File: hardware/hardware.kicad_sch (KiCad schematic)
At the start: 53 parts, among them J1 SWD, J2 serial, J3 analog, J4 digital_0, J5 digital_1, J6 digital_2, J7 digital_3, J8 power_0, J9 power_1, SW1 reset_btn, SW2 user_btn, SW3 SW_SPDT, U1 STM32F030CCTx, U2 AMS1117-3.3, Y1 crystal

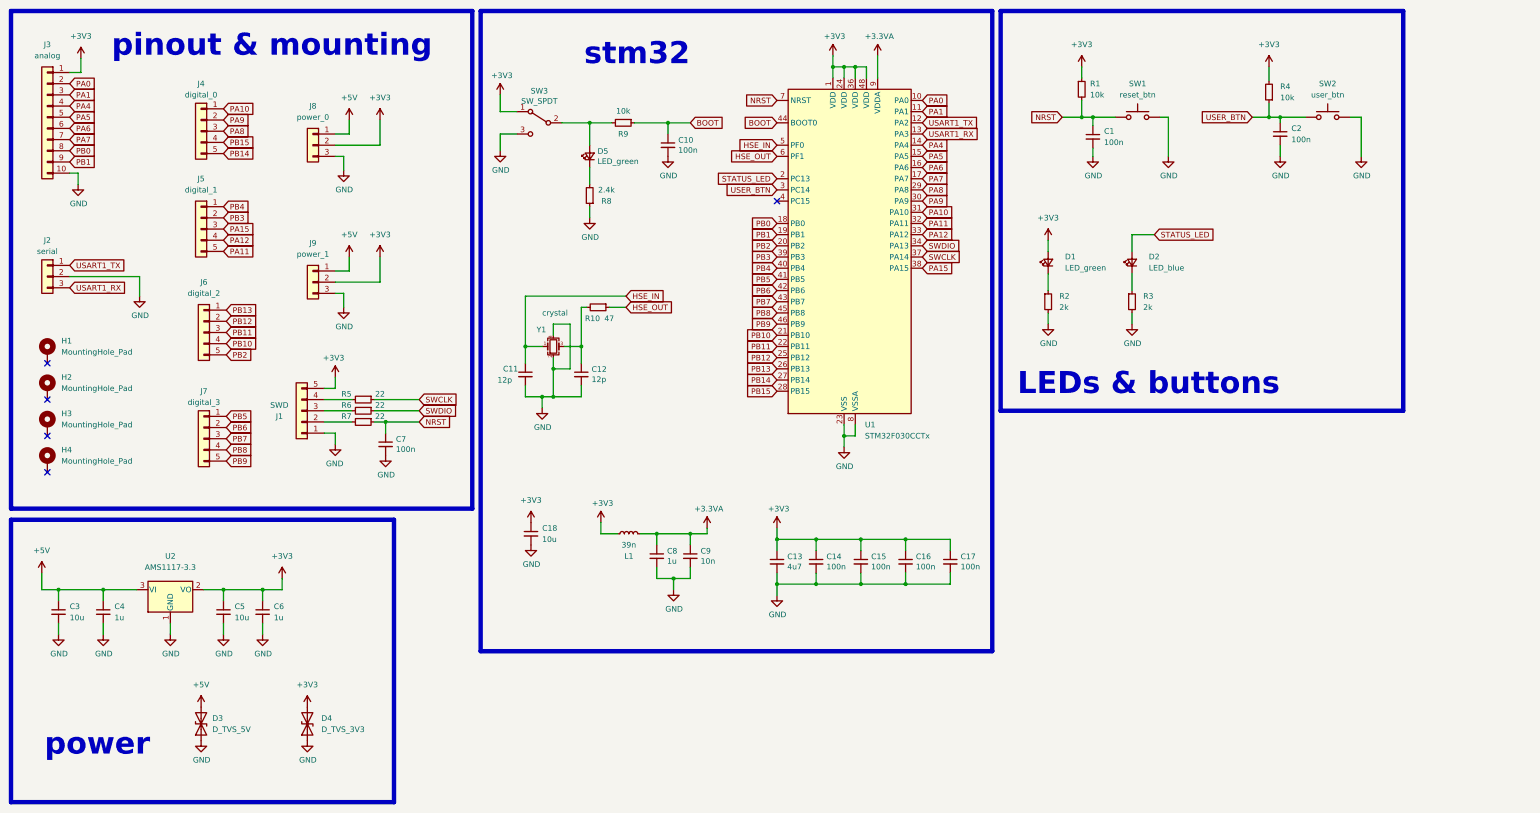
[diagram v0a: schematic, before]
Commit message: soldered and tested hardware
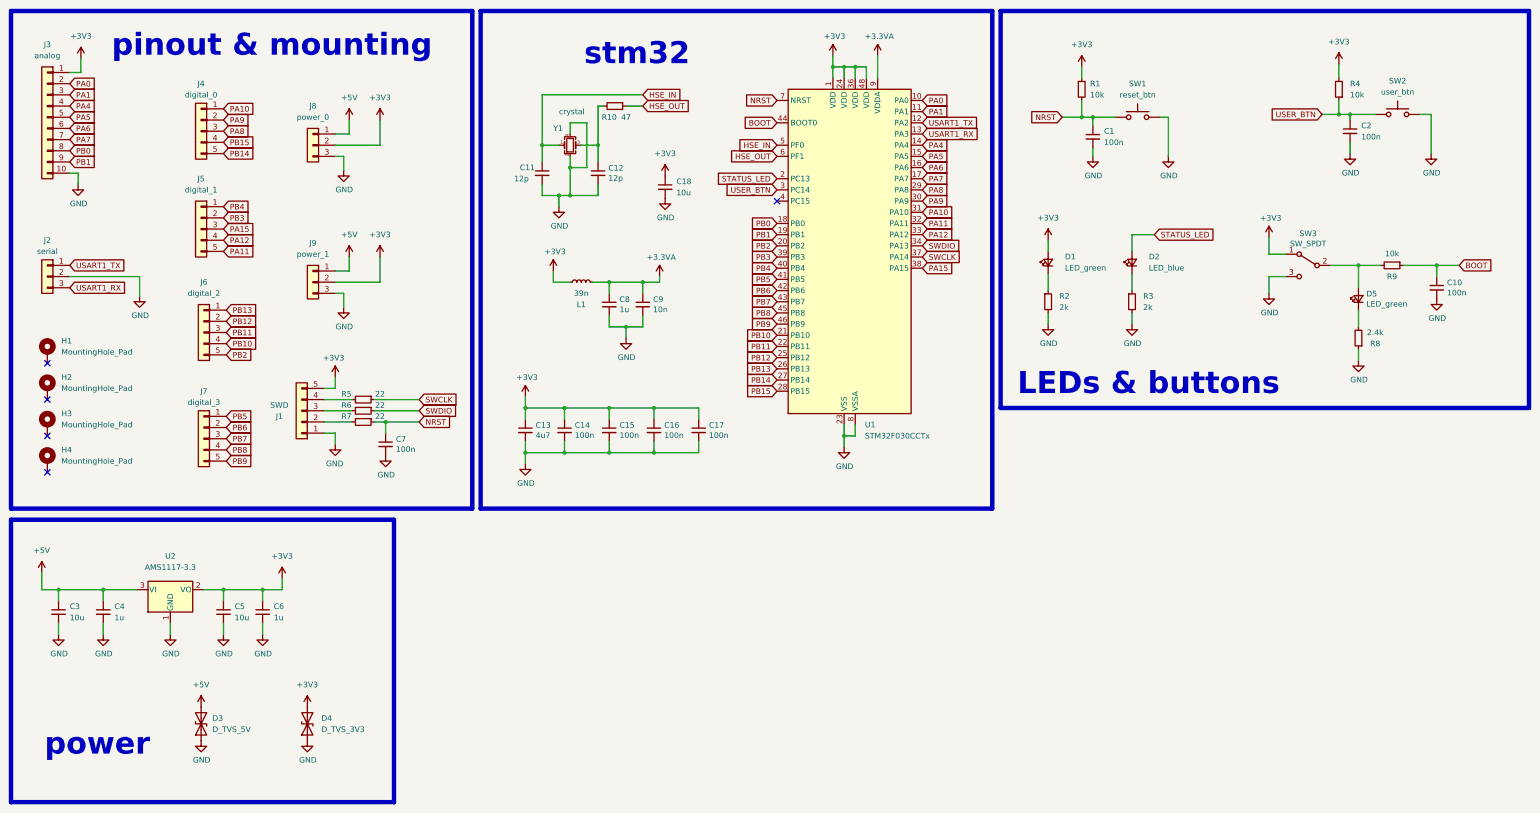
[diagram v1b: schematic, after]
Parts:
- C1, C2: LCSC part number C2857965 -> (none); in the shopping cart y -> (none)
- C10, C14, C15, C16, C17, C7: LCSC Part # C14663 -> (none); TODO OK -> (none); found (none) -> y
- C11, C12: LCSC Part # C182482 -> (none); TODO OK -> (none); found (none) -> y
- C13: LCSC Part # C19666 -> (none); TODO OK -> (none); found (none) -> y
- C18, C3, C5: LCSC part number C880609 -> (none); in the shopping cart y -> (none)
- C4: LCSC part number C2857985 -> (none); in the shopping cart y -> (none)
- C6: LCSC part number C967571 -> (none); in the shopping cart y -> (none)
- C8: LCSC Part # C15849 -> (none); TODO OK -> (none); found (none) -> y
- C9: LCSC Part # C57112 -> (none); TODO OK -> (none); found (none) -> y
- D1: LCSC part number C130722 -> (none); in the shopping cart y -> (none)
- D2: LCSC part number C130724 -> (none); in the shopping cart y -> (none)
- D3: LCSC part number C2892494 -> (none); found y -> (none); in the shopping cart y -> (none)
- D4: LCSC part number C316049 -> (none); found y -> (none); in the shopping cart y -> (none)
- D5: LCSC Part # C72043 -> (none); TODO OK -> (none); found (none) -> y
- L1: LCSC Part # C75654 -> (none); TODO OK -> (none); found (none) -> y
- R1, R4: LCSC part number C3015825 -> (none); in the shopping cart y -> (none)
- R10: LCSC Part # C23182 -> (none); TODO OK -> (none); found (none) -> y
- R2, R3: LCSC part number C3015799 -> (none); in the shopping cart y -> (none)
- R5, R6, R7: LCSC Part # C23345 -> (none); TODO OK -> (none); found (none) -> y
- R8: LCSC Part # C22940 -> (none); TODO OK -> (none); found (none) -> y
- R9: LCSC Part # C25804 -> (none); TODO OK -> (none); found (none) -> y
- SW1, SW2: LCSC part number C221897 -> (none); in the shopping cart y -> (none)
- SW3: TODO OK -> (none); found (none) -> y
- U1: found (none) -> y
- U2: in the shopping cart got it -> (none)
- Y1: LCSC Part # C13738 -> (none); TODO OK -> (none); found (none) -> y
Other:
- company: (none) -> Marcell Juhasz
- title: (none) -> CppCon 2024
- moved on the sheet: C10, C11, C12, C13, C14, C15, C16, C17, C18, C2, C8, C9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
